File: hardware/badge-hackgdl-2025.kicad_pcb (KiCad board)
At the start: 11 copper layers, 73.4 x 79.5 mm, 63 parts, among them J1 ADDON, J2 Battery, P1 USB_C_Plug_USB2.0, Q1 DMG3415U-7, Q2 MMBT2222A, SW1 ON, SW2 RESET, SW3 BOOT, SW4 RIGHT, SW5 BACK, SW6 LEFT, SW7 MIDDLE, U1 XC6220B331MR-G, U2 ESP32-S3-WROOM-1-N16

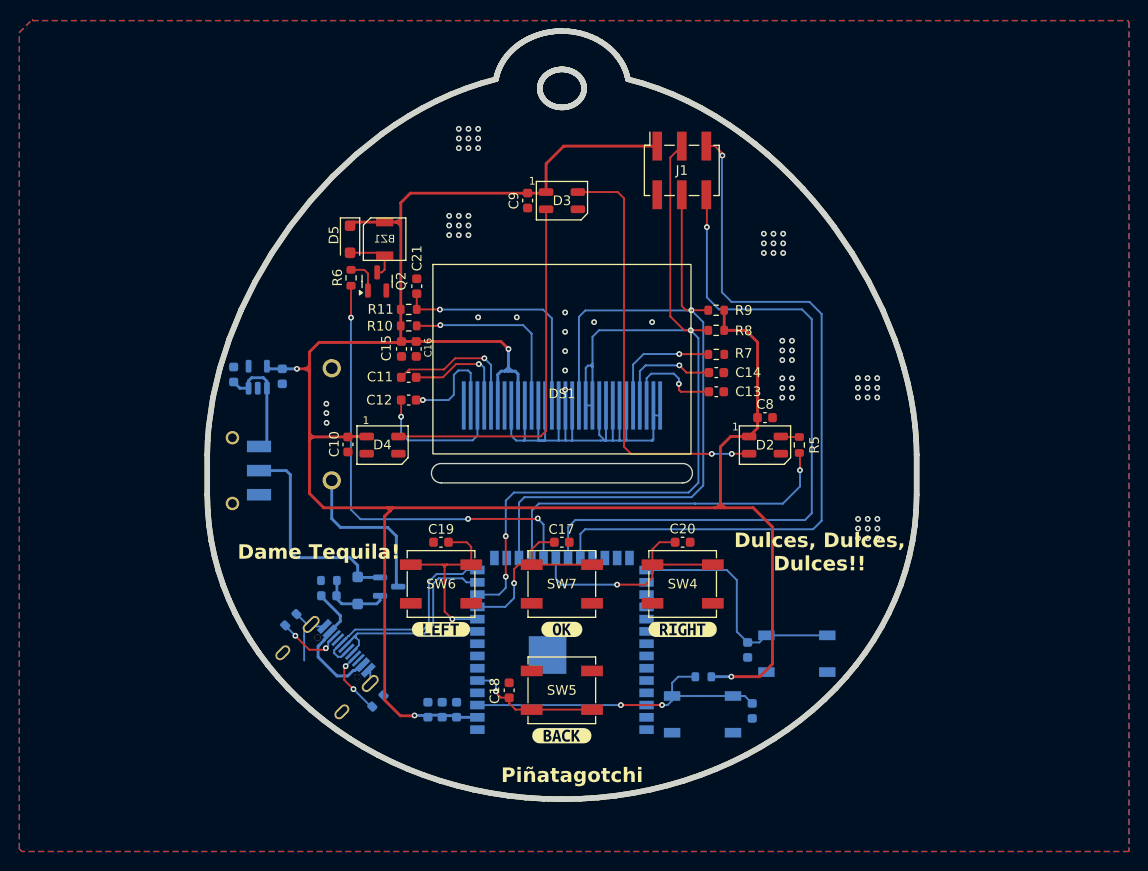
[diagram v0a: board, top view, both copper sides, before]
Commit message: feat(hw): add 3d model for pcb
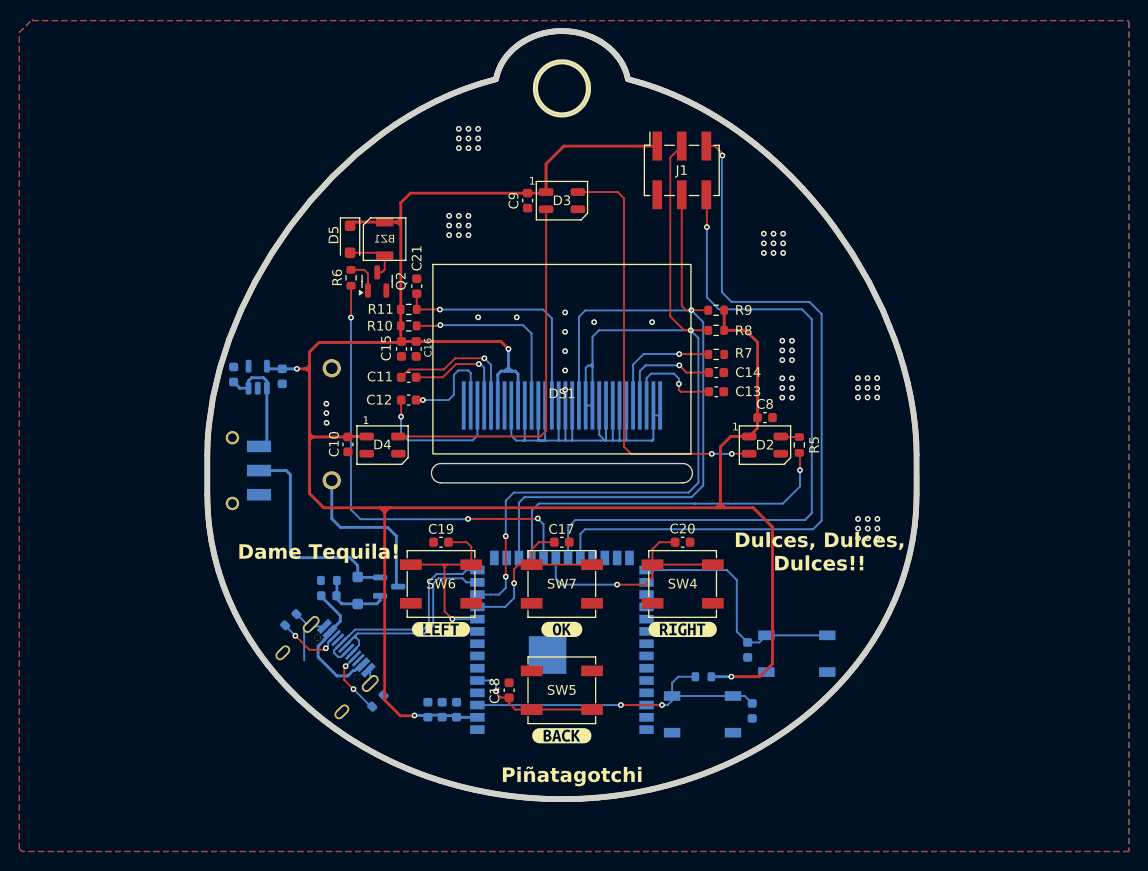
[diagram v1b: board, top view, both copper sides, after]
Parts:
- added Ref** (x2): Val**, Footprints:badge-hackgdl-2025-Edge_Cuts, F.Cu at (133.7, 58.6)
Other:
- outline, holes or cut-outs redrawn
